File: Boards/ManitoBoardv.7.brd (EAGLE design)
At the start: 75.2 x 64.8 mm, 43 parts, among them U1 BLUETOOTH-RN41", U2 ATMEGA328P

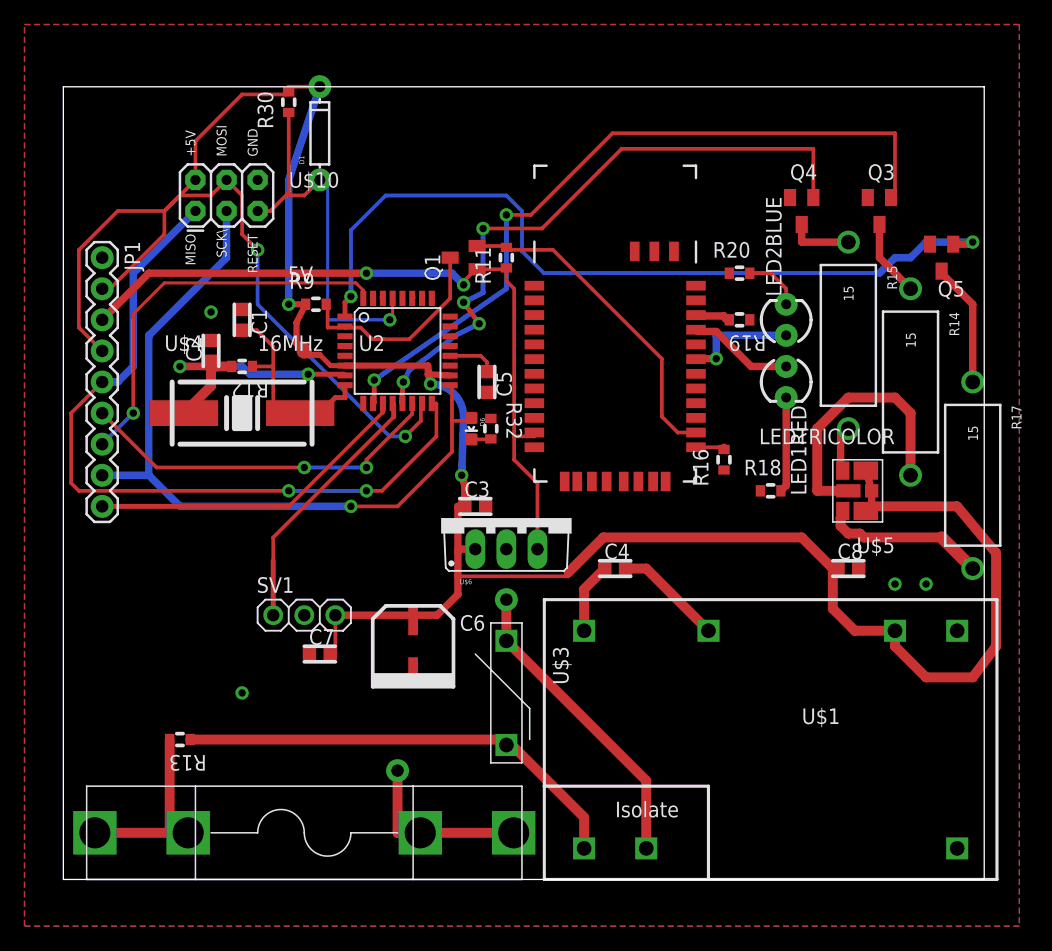
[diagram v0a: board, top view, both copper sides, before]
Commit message: Fixed Layout Issues
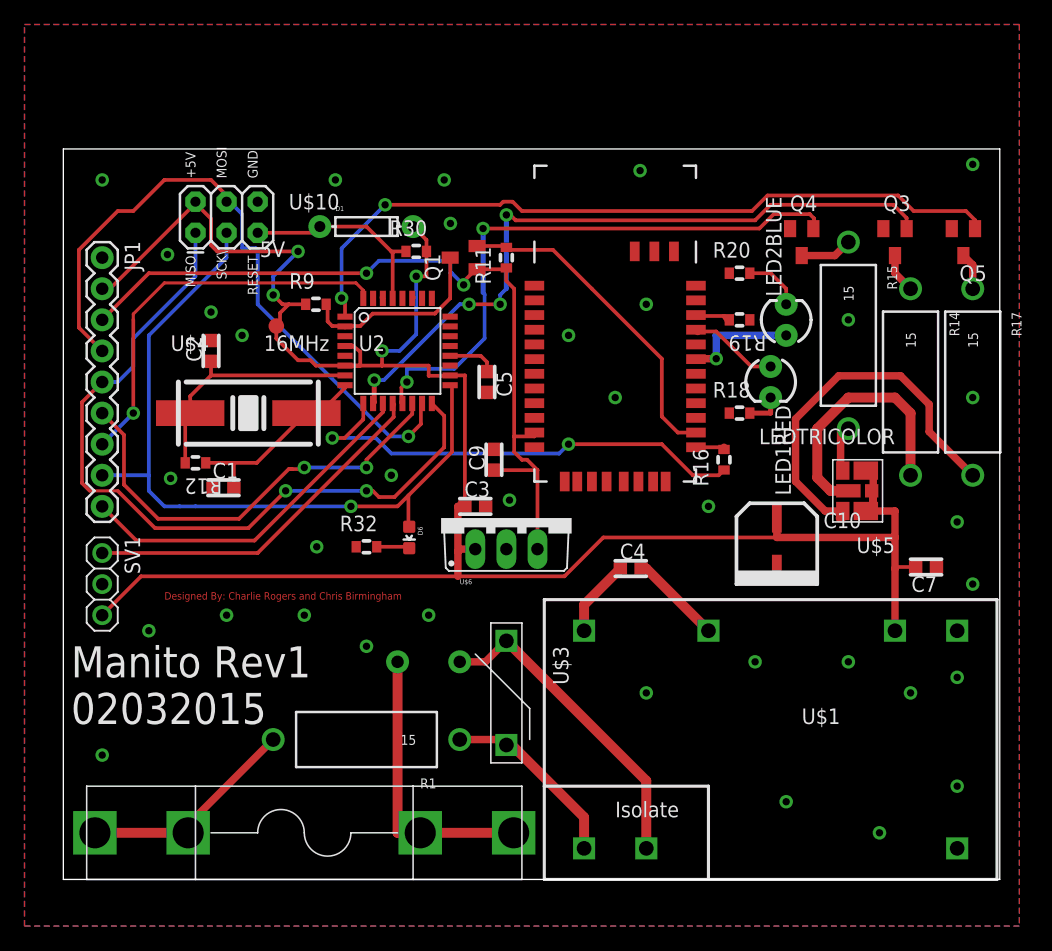
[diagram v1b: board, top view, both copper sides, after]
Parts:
- removed C6: 100u, CharlieCreations:WXSERIES-SMDCAP
- removed C8: 100u, CharlieCreations:0603-CAP
- removed R13: 10, CharlieCreations:0603RESISTOR
- added C10: 100u, CharlieCreations:WXSERIES-SMDCAP
- added C9: 4.7u, CharlieCreations:0603-CAP
- added R1: 15, SparkFun-Passives:AXIAL-0.6
- moved C7 50.0 mm to (92.7, 29.3), turned to 180 degrees
- moved SV1 16.7 mm to (25.4, 27.9), turned to 270 degrees
- moved R30 16.0 mm to (51.1, 55.1), turned to 0 degrees
- moved R32 14.0 mm to (47.0, 31.0), turned to 0 degrees
- moved C1 13.8 mm to (35.3, 35.8), turned to 0 degrees
- moved D6 10.2 mm to (50.5, 31.8)
- moved LINE 8.89 mm to (49.5, 21.6)
- moved R12 8.75 mm to (33.0, 37.8)
- moved D1 8.52 mm to (47.0, 57.1), turned to 0 degrees
- moved R17 7.62 mm to (96.5, 44.5)
- moved R18 6.84 mm to (77.5, 41.9)
- moved NEUTRAL 6.35 mm to (54.6, 21.6)
- moved 5V 3.06 mm to (39.6, 49.0)
- moved Q3 2.84 mm to (90.2, 55.9)
- moved Q4 2.54 mm to (82.5, 55.9)
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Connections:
- net +5V: now also C10.POS; no longer C6.POS, C8.1
- net GND: now also C10.NEG, C9.2; no longer C6.NEG, C8.2
- net N$22: now also R1.P$1; no longer R13.1
- net N$25: now also R1.P$2; no longer R13.2
- net VCC: now also C9.1
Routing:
- net IO5/RX: track 0.00 -> 38.5 mm, vias 0 -> 2
- net N$22: track 37.6 -> 15.8 mm
- net N$31: track 13.5 -> 31.2 mm
- net RESET: track 32.2 -> 17.0 mm, vias 1 -> 0
- net N$24: track 14.6 -> 23.5 mm
- net IO8/PIR_SIG: track 21.4 -> 29.6 mm
- net N$6: track 10.1 -> 3.03 mm
- net IO10/SS: track 30.2 -> 35.9 mm
- net VCC: track 62.1 -> 67.3 mm
- net IO3: track 66.5 -> 61.4 mm
- net N$3: track 7.80 -> 2.97 mm
- net IO9: track 52.6 -> 48.0 mm, vias 4 -> 2
- net IO6: track 61.2 -> 57.0 mm, vias 2 -> 4
- net +5V: track 179.1 -> 175.5 mm, vias 3 -> 4
- net N$4: track 23.5 -> 20.3 mm, vias 2 -> 0
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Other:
- board size 75.2 x 64.8 mm -> 76.5 x 59.7 mm
- board text added: "02032015"
- board text added: "Designed By: Charlie Rogers and Chris Birmingham"
- board text added: "Manito Rev1"
